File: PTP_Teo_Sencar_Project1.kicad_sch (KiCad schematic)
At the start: 25 parts, among them J1 Screw_Terminal_01x02, SW1 SW_Push, SW2 SW_SPDT_312, U1 LM2574N-5, U5 NE555P, U6 74LVC1G11

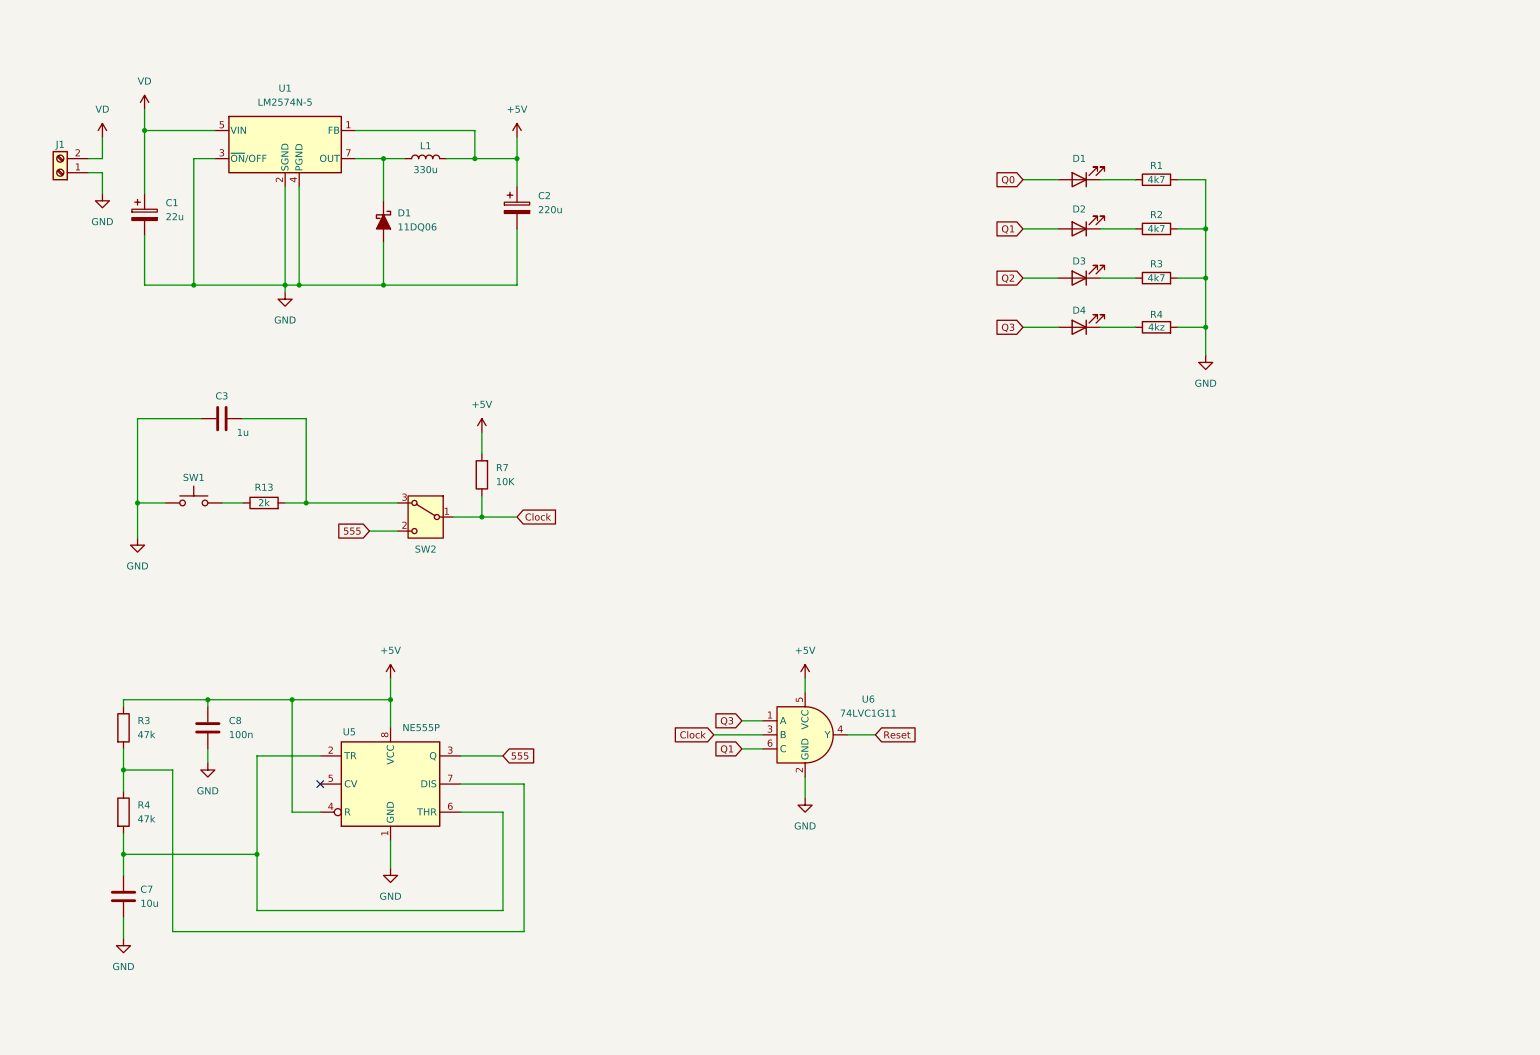
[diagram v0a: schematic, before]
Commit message: Popunjeni parametri komponenata
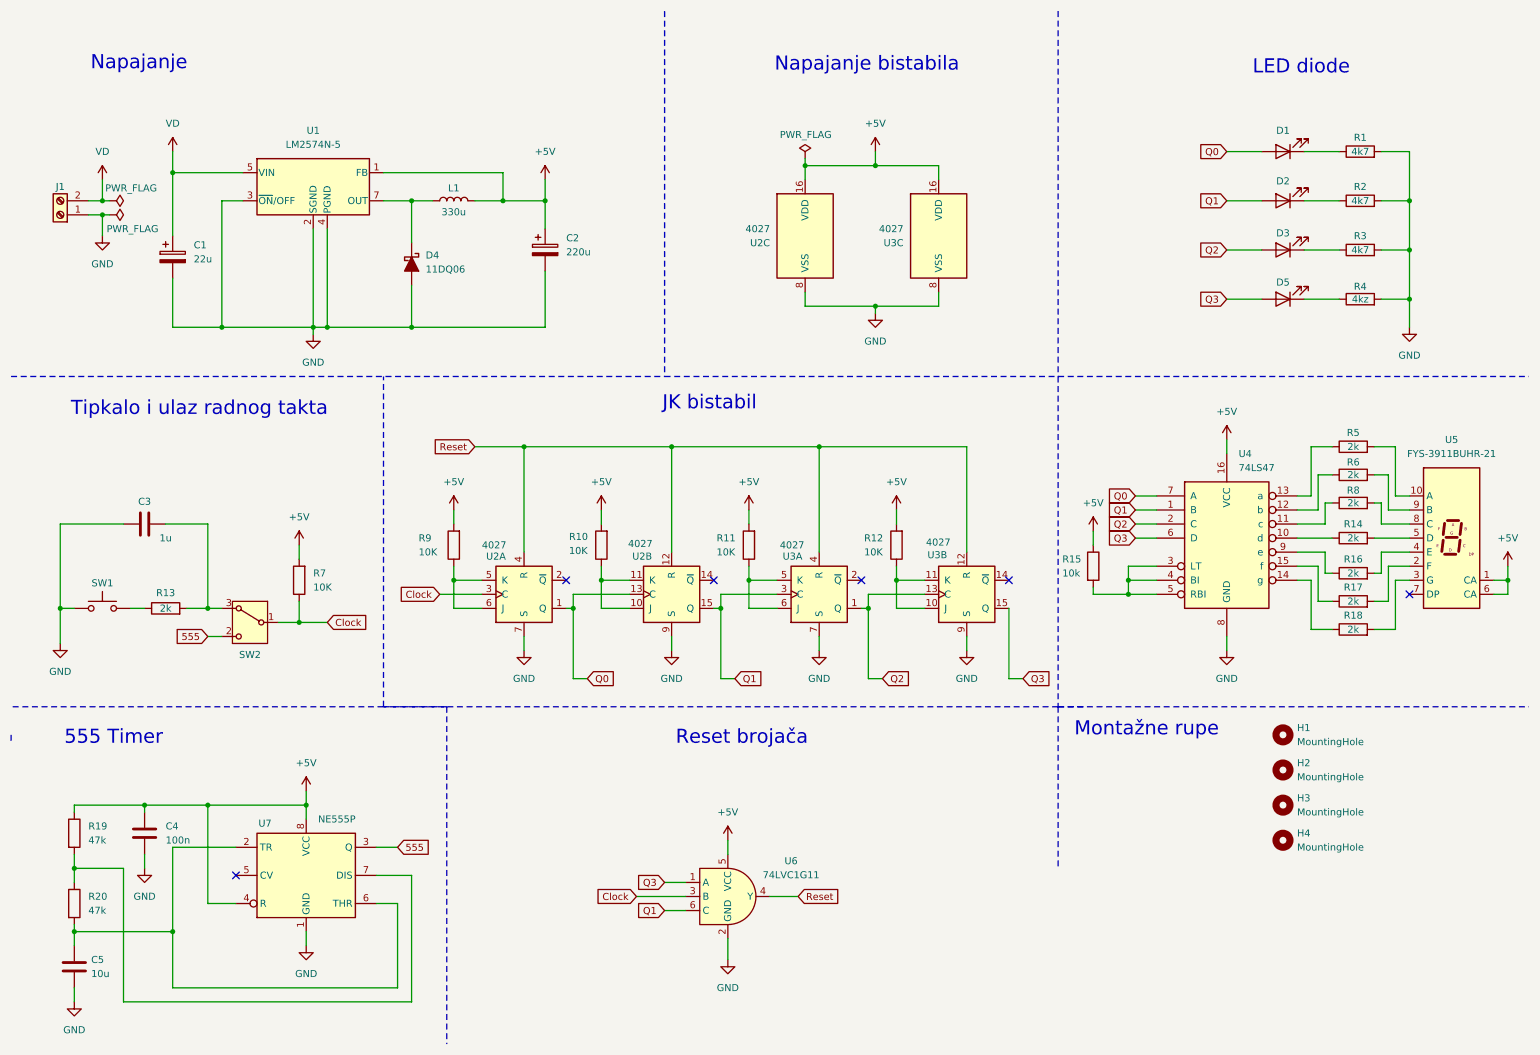
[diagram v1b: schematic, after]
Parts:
- added H1, H2, H3, H4: MountingHole, symbol Mechanical:MountingHole
- added R10, R11, R12, R9: 10K, symbol Device:R
- added R14, R16, R17, R18, R5, R6, R8: 2k, symbol Device:R
- added R15: 10k, symbol Device:R
- added U2, U3: 4027, symbol 4xxx:4027
- added U4: 74LS47, symbol 74xx:74LS47
- added U5: FYS-3911BUHR-21, Display_7Segment:HDSP-7401, symbol Display_Character:HDSP-7401
- C1: footprint (none) -> Capacitor_THT:CP_Radial_D5.0mm_P2.00mm; Manufacturer (none) -> AISHI; Manufacturer Part Number (none) -> EWH1EM220D11OT
- C2: footprint (none) -> Capacitor_THT:CP_Radial_D5.0mm_P2.00mm; Manufacturer (none) -> SAMWHA; Manufacturer Part Number (none) -> RD1A227M05011BB
- C3: footprint (none) -> Capacitor_SMD:C_1206_3216Metric_Pad1.33x1.80mm_HandSolder; Manufacturer (none) -> SAMSUNG; Manufacturer Part Number (none) -> CL31B105KBHNNNE
- C4: renamed from C8; footprint (none) -> Capacitor_SMD:C_1206_3216Metric_Pad1.33x1.80mm_HandSolder; Manufacturer (none) -> SAMSUNG; Manufacturer Part Number (none) -> CL31B104KBCNNNC
- C5: renamed from C7; footprint (none) -> Capacitor_SMD:C_1206_3216Metric_Pad1.33x1.80mm_HandSolder; Manufacturer (none) -> SAMSUNG; Manufacturer Part Number (none) -> CL31A106KBHNNNE
- D1, D2, D3: footprint (none) -> LED_THT:LED_D5.0mm
- D4: renamed from D1; footprint (none) -> Diode_THT:D_DO-41_SOD81_P12.70mm_Horizontal; Manufacturer (none) -> SMC DIODE SOLUTIONS; Manufacturer Part Number (none) -> 11DQ06TA
- D5: renamed from D4; footprint (none) -> LED_THT:LED_D5.0mm
- renumbered R3 to R19, R4 to R20, U5 to U7
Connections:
- net +5V: now also R10.2, R11.2, R12.2, R15.1, R9.2, U2.16 (VDD), U3.16 (VDD), U4.16 (VCC), U5.1 (CA), U5.6 (CA)
- net Clock: now also U2.3 (C)
- net GND: now also U2.7 (S), U2.8 (VSS), U2.9 (S), U3.7 (S), U3.8 (VSS), U3.9 (S), U4.8 (GND)
- net Q0: now also U2.1 (Q), U2.13 (C), U4.7 (A)
- net Q1: now also U2.15 (Q), U3.3 (C), U4.1 (B)
- net Q2: now also U3.1 (Q), U3.13 (C), U4.2 (C)
- net Q3: now also U3.15 (Q), U4.6 (D)
- net Reset: now also U2.12 (R), U2.4 (R), U3.12 (R), U3.4 (R)
- new net: R6.1, U4.12 (b)
- new net: R6.2, U5.9 (B)
- new net: R5.2, U5.10 (A)
- new net: R17.2, U5.2 (F)
- new net: R18.2, U5.3 (G)
- new net: R16.2, U5.4 (E)
- new net: R14.2, U5.5 (D)
- new net: R8.2, U5.8 (C)
- new net: R15.2, U4.3 (LT), U4.4 (BI), U4.5 (RBI)
- new net: R12.1, U3.10 (J), U3.11 (K)
- new net: R5.1, U4.13 (a)
- new net: R16.1, U4.9 (e)
- new net: R10.1, U2.10 (J), U2.11 (K)
- new net: R18.1, U4.14 (g)
- new net: R14.1, U4.10 (d)
- new net: R17.1, U4.15 (f)
- new net: R11.1, U3.5 (K), U3.6 (J)
- new net: R9.1, U2.5 (K), U2.6 (J)
- new net: R8.1, U4.11 (c)
- no-connect marks 1 -> 6
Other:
- note added: "555 Timer"
- note added: "JK bistabil"
- note added: "LED diode"
- note added: "Montažne rupe"
- note added: "Napajanje"
- note added: "Napajanje bistabila"
- note added: "Reset brojača"
- note added: "Tipkalo i ulaz radnog takta"
- moved on the sheet: C1, C2, C3, C4, C5, D1, D2, D3, D4, D5, J1, L1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
